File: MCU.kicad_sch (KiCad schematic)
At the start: 28 parts, among them J2 USB_C_Receptacle_USB2.0_16P, J8 FTSH-105-01-L-DV-K-A, U1 STM32H743VITx, Y1 Crystal_GND24

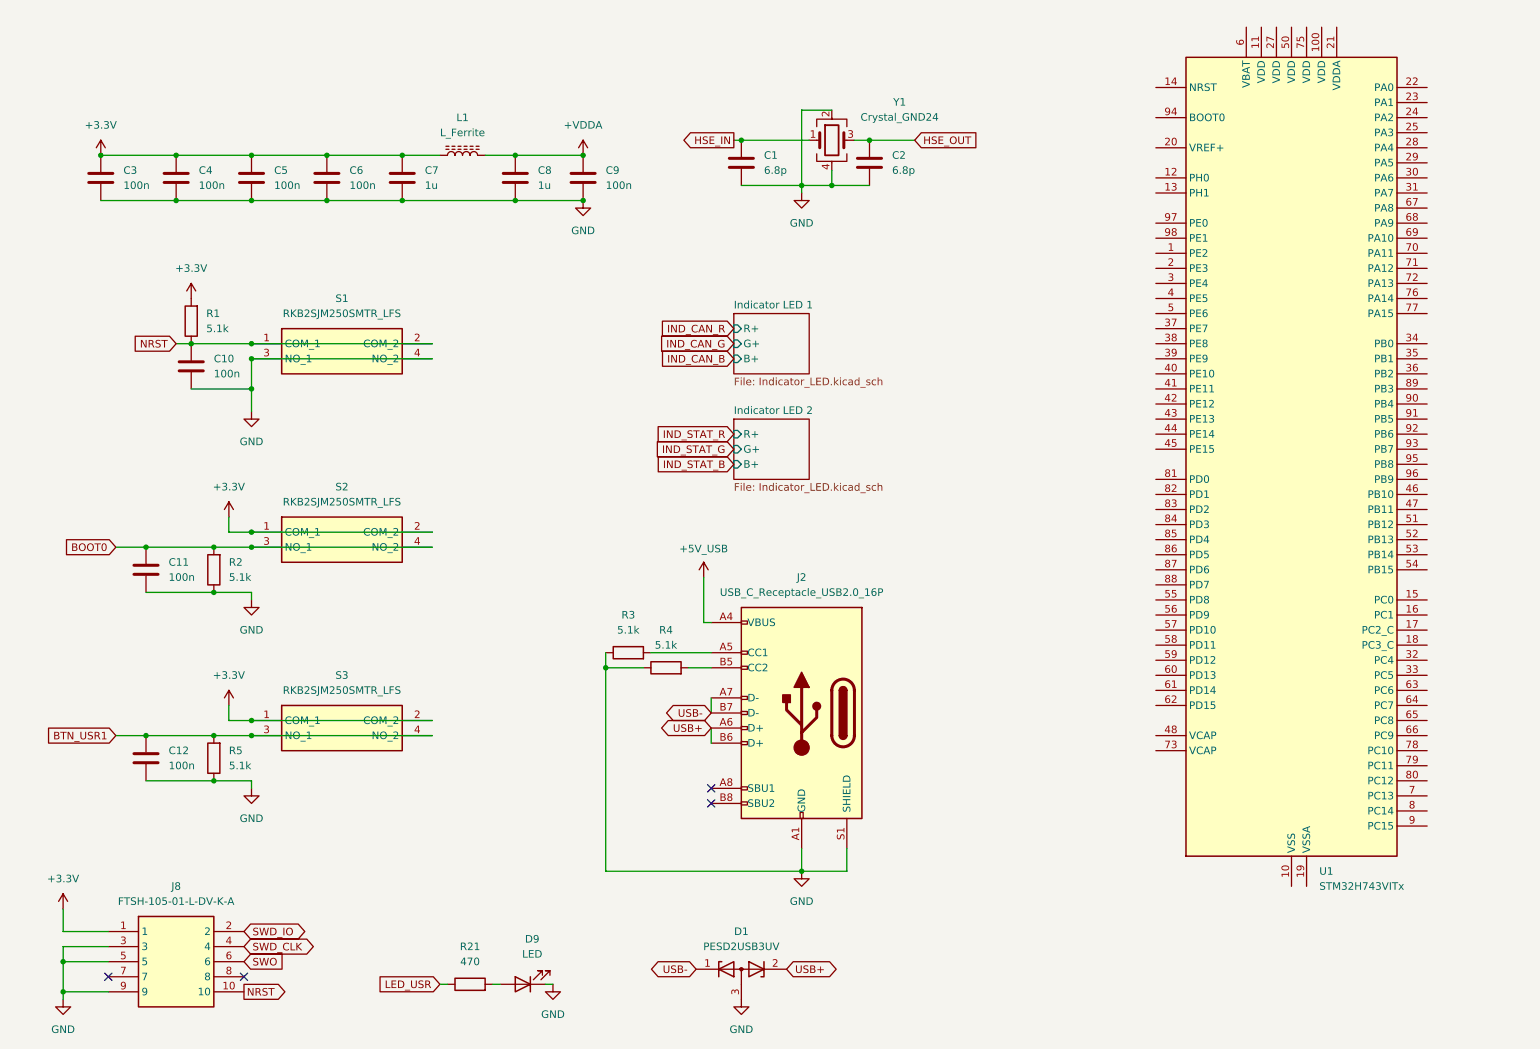
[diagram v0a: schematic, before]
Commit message: LCD connector, backlight, other work
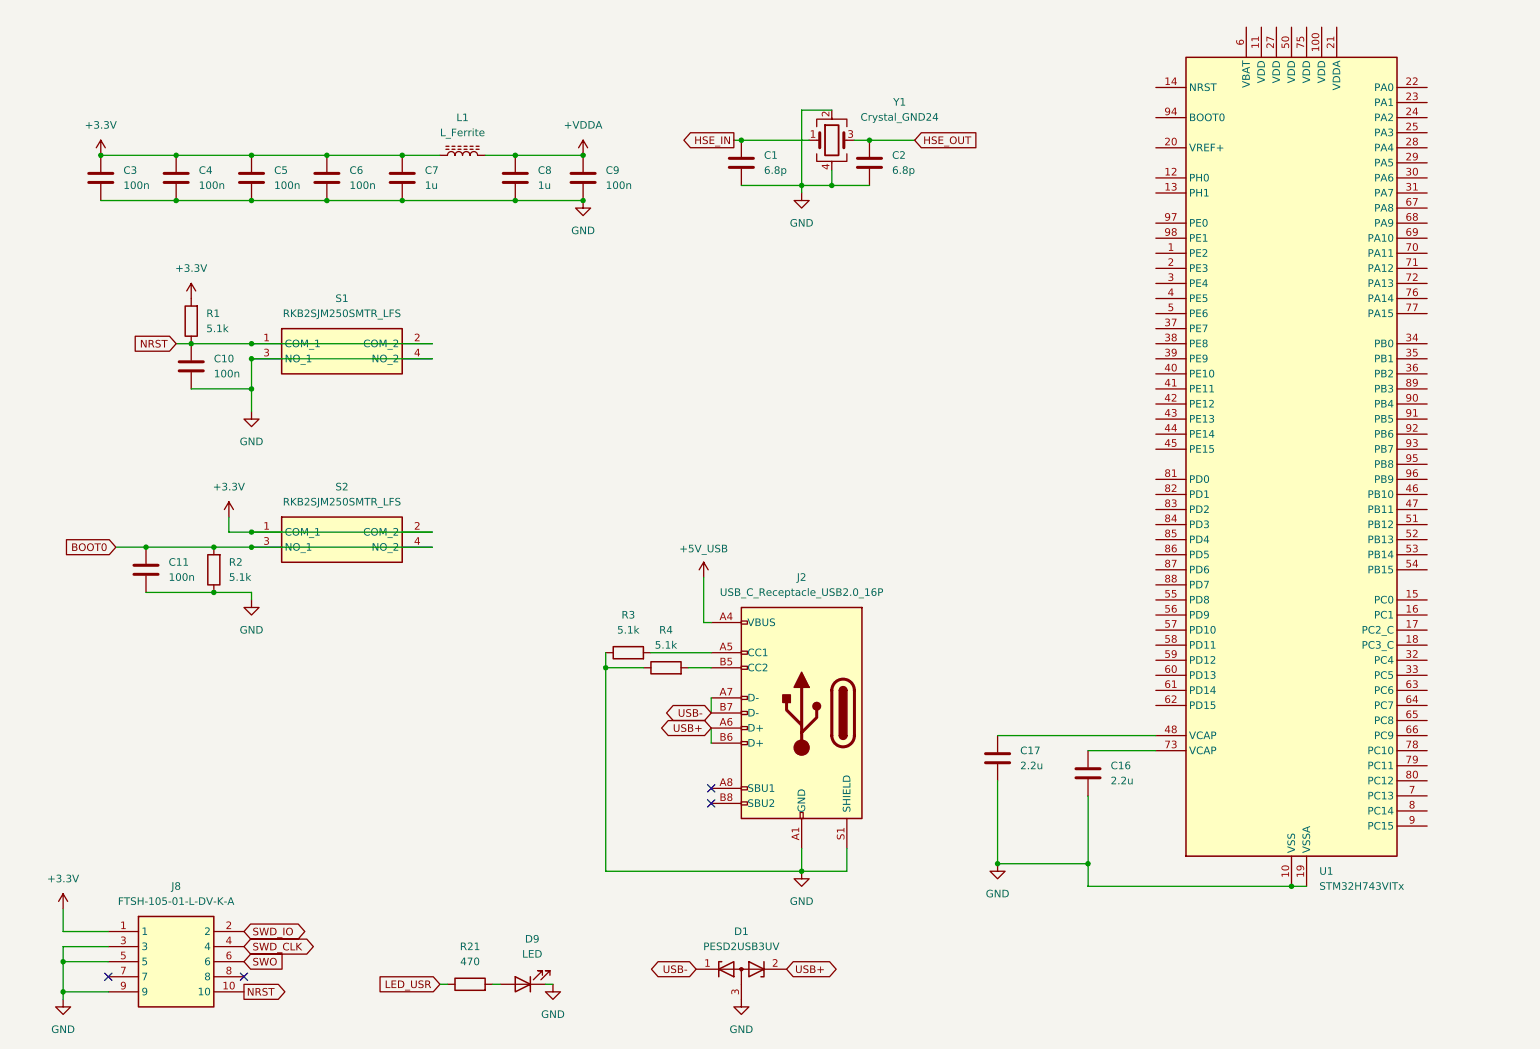
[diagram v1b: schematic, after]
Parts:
- removed C12: 100n, Capacitor_SMD:C_0603_1608Metric_Pad1.08x0.95mm_HandSolder, symbol Device:C
- removed R5: 5.1k, Resistor_SMD:R_0603_1608Metric_Pad0.98x0.95mm_HandSolder, symbol Device:R
- removed S3: RKB2SJM250SMTR_LFS, RKB2SJM250SMTRLFS, symbol SamacSys_Parts:RKB2SJM250SMTR_LFS
- added C16, C17: 2.2u, Capacitor_SMD:C_0603_1608Metric_Pad1.08x0.95mm_HandSolder, symbol Device:C
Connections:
- net GND: now also U1.10 (VSS), U1.19 (VSSA), U1.26 (VSS), U1.49 (VSS), U1.74 (VSS), U1.99 (VSS), C16.2, C17.2
- net at U1.48 (VCAP): now also C17.1
- net at U1.73 (VCAP): now also C16.1
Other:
- removed sheet Indicator LED 1
- removed sheet Indicator LED 2

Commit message: preliminary complete schematic
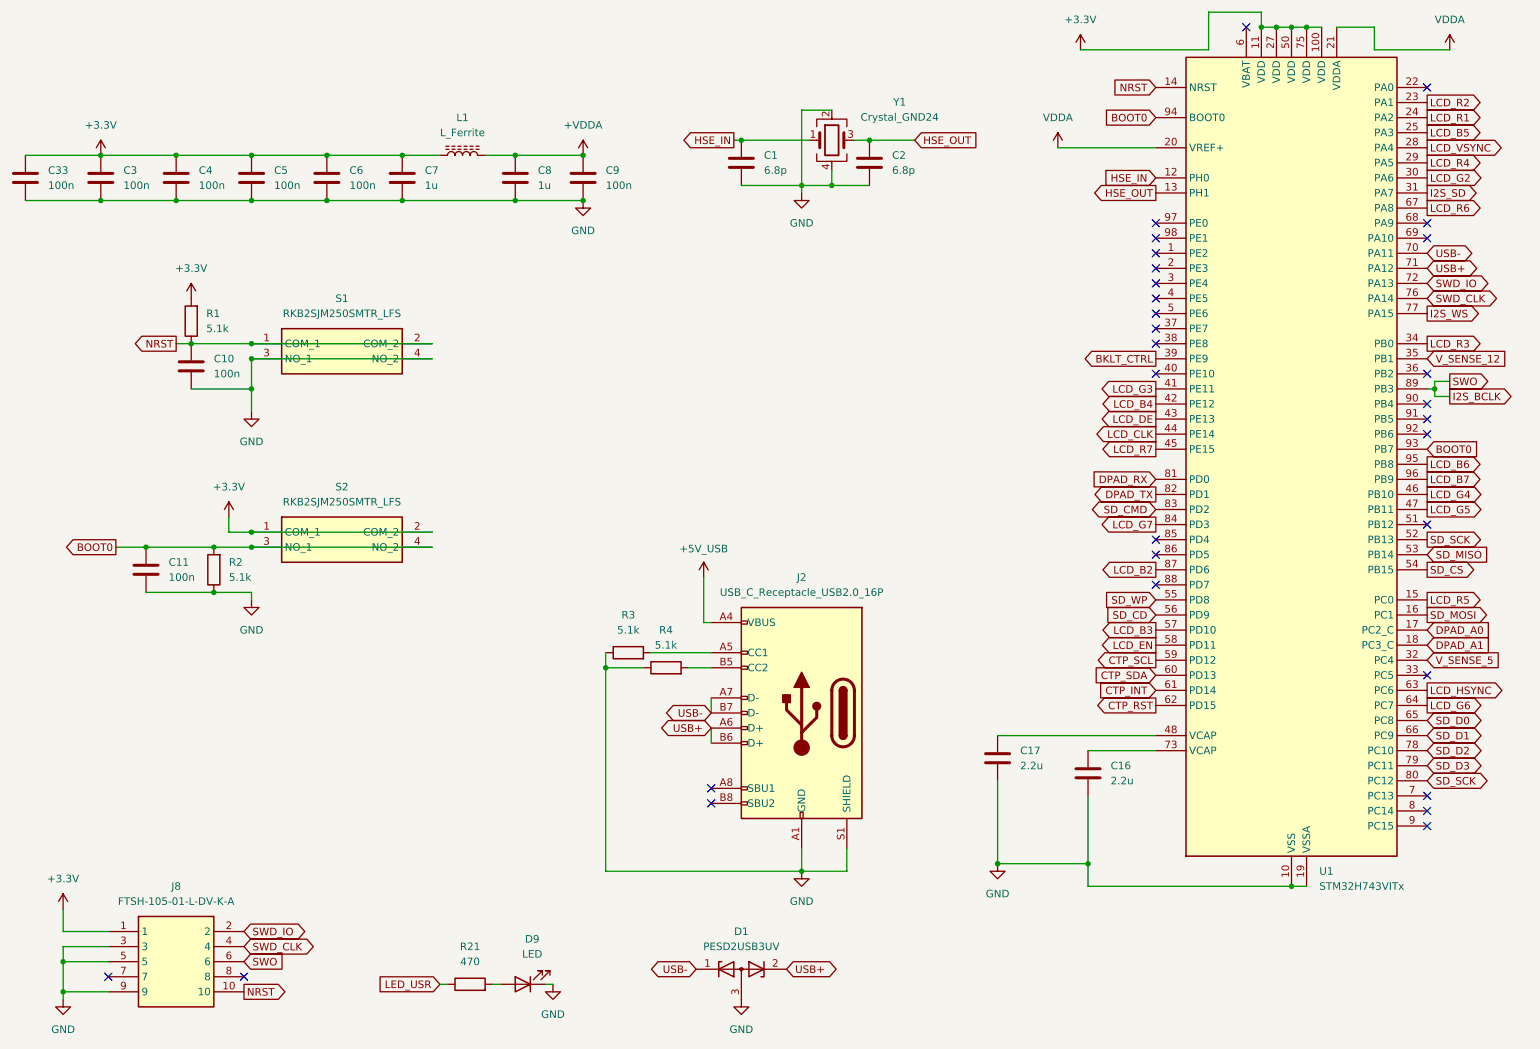
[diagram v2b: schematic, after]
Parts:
- added C33: 100n, Capacitor_SMD:C_0603_1608Metric_Pad1.08x0.95mm_HandSolder, symbol Device:C
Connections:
- net SWO is gone; now on net I2S_BCLK: J8.6
- net +3.3V: now also U1.100 (VDD), U1.11 (VDD), U1.27 (VDD), U1.50 (VDD), U1.75 (VDD), C33.1
- net BOOT0: now also U1.93 (PB7), U1.94 (BOOT0)
- net GND: now also C33.2
- net HSE_IN: now also U1.12 (PH0)
- net HSE_OUT: now also U1.13 (PH1)
- net NRST: now also U1.14 (NRST)
- net SWD_CLK: now also U1.76 (PA14)
- net SWD_IO: now also U1.72 (PA13)
- net USB+: now also U1.71 (PA12)
- net USB-: now also U1.70 (PA11)
- net LCD_R5: now reaches U1.15 (PC0)
- net SD_MOSI: now reaches U1.16 (PC1)
- net DPAD_A0: now reaches U1.17 (PC2_C)
- net DPAD_A1: now reaches U1.18 (PC3_C)
- net VDDA: now reaches U1.20 (VREF+)
- net VDDA: now also U1.21 (VDDA)
- net LCD_R2: now reaches U1.23 (PA1)
- net LCD_R1: now reaches U1.24 (PA2)
- net LCD_B5: now reaches U1.25 (PA3)
- net LCD_VSYNC: now reaches U1.28 (PA4)
- net LCD_R4: now reaches U1.29 (PA5)
- net LCD_G2: now reaches U1.30 (PA6)
- net I2S_SD: now reaches U1.31 (PA7)
- net V_SENSE_5: now reaches U1.32 (PC4)
- net LCD_R3: now reaches U1.34 (PB0)
- net V_SENSE_12: now reaches U1.35 (PB1)
- net BKLT_CTRL: now reaches U1.39 (PE9)
- net LCD_G3: now reaches U1.41 (PE11)
- net LCD_B4: now reaches U1.42 (PE12)
- net LCD_DE: now reaches U1.43 (PE13)
- net LCD_CLK: now reaches U1.44 (PE14)
- net LCD_R7: now reaches U1.45 (PE15)
- net LCD_G4: now reaches U1.46 (PB10)
- net LCD_G5: now reaches U1.47 (PB11)
- net SD_SCK: now reaches U1.52 (PB13)
- net SD_SCK: now also U1.80 (PC12)
- net SD_MISO: now reaches U1.53 (PB14)
- net SD_CS: now reaches U1.54 (PB15)
- net SD_WP: now reaches U1.55 (PD8)
- net SD_CD: now reaches U1.56 (PD9)
- net LCD_B3: now reaches U1.57 (PD10)
- net LCD_EN: now reaches U1.58 (PD11)
- net CTP_SCL: now reaches U1.59 (PD12)
- net CTP_SDA: now reaches U1.60 (PD13)
- net CTP_INT: now reaches U1.61 (PD14)
- net CTP_RST: now reaches U1.62 (PD15)
- net LCD_HSYNC: now reaches U1.63 (PC6)
- net LCD_G6: now reaches U1.64 (PC7)
- net SD_D0: now reaches U1.65 (PC8)
- net SD_D1: now reaches U1.66 (PC9)
- net LCD_R6: now reaches U1.67 (PA8)
- net I2S_WS: now reaches U1.77 (PA15)
- net SD_D2: now reaches U1.78 (PC10)
- net SD_D3: now reaches U1.79 (PC11)
- net DPAD_RX: now reaches U1.81 (PD0)
- net DPAD_TX: now reaches U1.82 (PD1)
- net SD_CMD: now reaches U1.83 (PD2)
- net LCD_G7: now reaches U1.84 (PD3)
- net LCD_B2: now reaches U1.87 (PD6)
- net I2S_BCLK: now reaches U1.89 (PB3)
- net LCD_B6: now reaches U1.95 (PB8)
- net LCD_B7: now reaches U1.96 (PB9)
- no-connect marks 4 -> 30
